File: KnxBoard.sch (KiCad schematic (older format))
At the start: 9 parts, among them J1 SB, J2 KNX, J3 Conn_01x14, J4 Conn_01x02, J5 Conn_01x14, SW1 SW

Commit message: Resistors in 0402
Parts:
- R1: footprint Resistor_SMD:R_0603_1608Metric -> Resistor_SMD:R_0402_1005Metric
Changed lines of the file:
@@
 F 0 "R1" H 2670 1246 50  0000 L CNN
 F 1 "100R" H 2670 1155 50  0000 L CNN
-F 2 "Resistor_SMD:R_0603_1608Metric" V 2530 1200 50  0001 C CNN
-F 3 "https://www.mouser.fr/ProductDetail/Vishay-Dale/CRCW0603100RFKEAC?qs=sGAEpiMZZMvdGkrng054t0DrEhLhGh8gD13mKavhucb20%2FizL9tlHg%3D%3D" H 2600 1200 50  0001 C CNN
+F 2 "Resistor_SMD:R_0402_1005Metric" V 2530 1200 50  0001 C CNN
+F 3 "https://www.mouser.fr/ProductDetail/Vishay-Dale/CRCW0402100RFKEDC?qs=sGAEpiMZZMvdGkrng054t0DrEhLhGh8gJaf4W6KCPV2ghVtyILDy9w%3D%3D" H 2600 1200 50  0001 C CNN
 F 4 "0.09" H 2600 1200 50  0001 C CNN "Price"
 	1    2600 1200

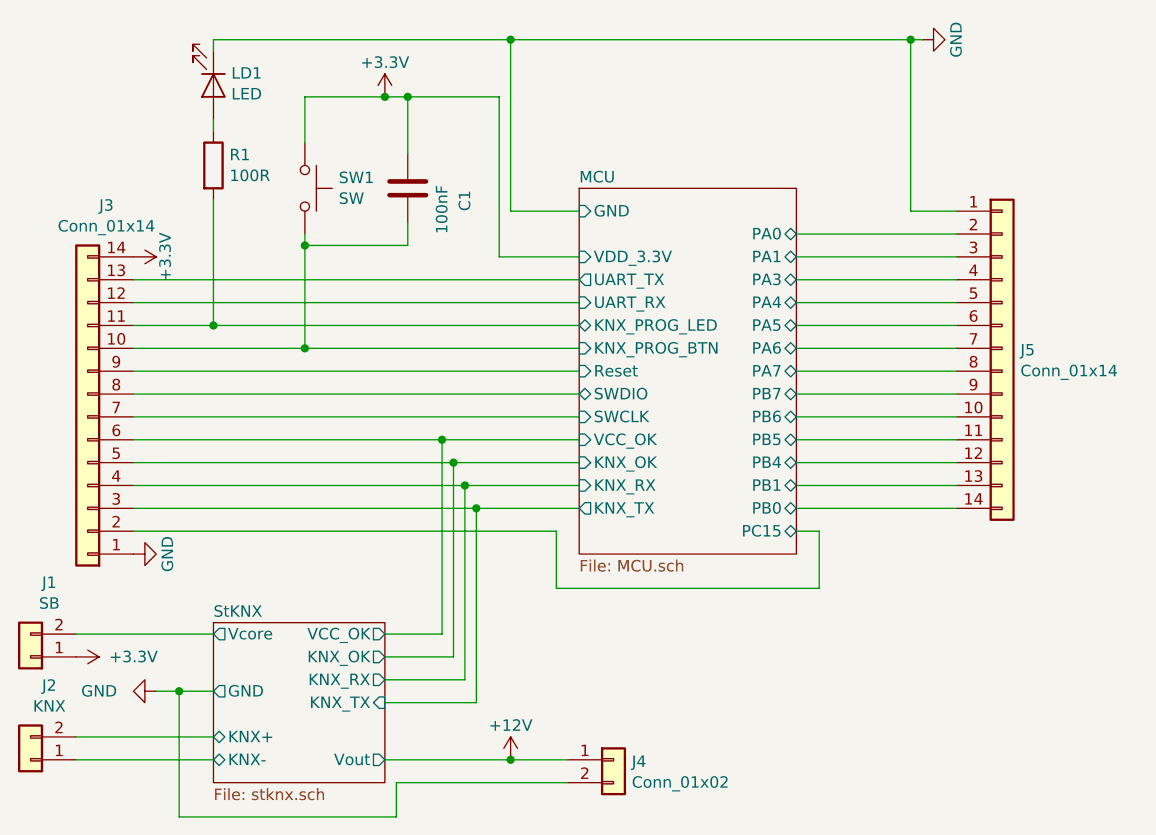
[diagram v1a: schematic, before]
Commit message: Update
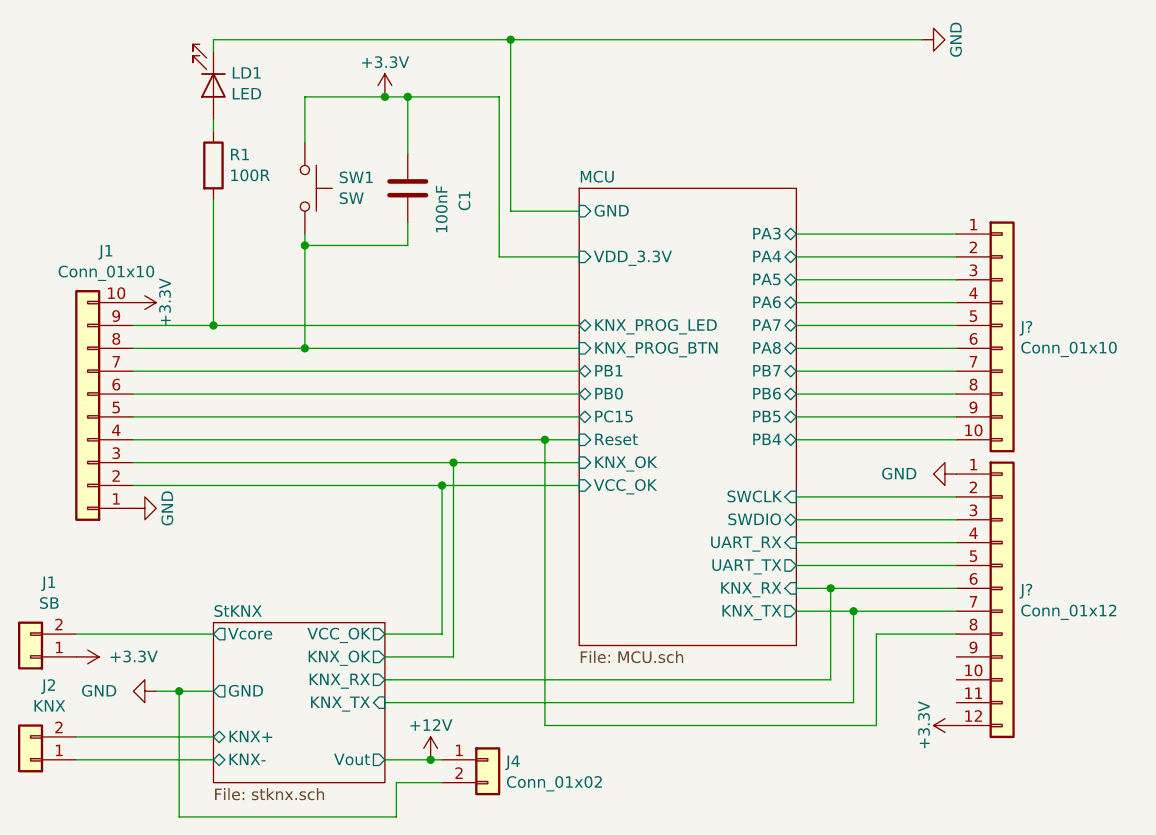
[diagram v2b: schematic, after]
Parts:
- removed J3, J5: Conn_01x14, Connector_PinHeader_2.54mm:PinHeader_1x14_P2.54mm_Vertical, symbol Connector_Generic:Conn_01x14
- added J1: Conn_01x10, Connector_PinHeader_2.54mm:PinHeader_1x14_P2.54mm_Vertical, symbol Connector_Generic:Conn_01x10
- added J?: Conn_01x12, Connector_FFC-FPC:Hirose_FH12-12S-0.5SH_1x12-1MP_P0.50mm_Horizontal, symbol Connector_Generic:Conn_01x12
- added J?: Conn_01x10, symbol Connector_Generic:Conn_01x10
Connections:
- net +3V3: now also J1.10 (Pin_10), J?.12 (Pin_12)
- net GND: now also J1.1 (Pin_1), J?.1 (Pin_1)
- net MCU/KNX_OK: now also J1.3 (Pin_3)
- net MCU/KNX_PROG_BTN: now also J1.8 (Pin_8)
- net MCU/KNX_PROG_LED: now also J1.9 (Pin_9)
- net MCU/KNX_RX: now also J?.6 (Pin_6)
- net MCU/KNX_TX: now also J?.7 (Pin_7)
- net MCU/PA3: now also J?.1 (Pin_1)
- net MCU/PA4: now also J?.2 (Pin_2)
- net MCU/PA5: now also J?.3 (Pin_3)
- net MCU/PA6: now also J?.4 (Pin_4)
- net MCU/PA7: now also J?.5 (Pin_5)
- net MCU/PB0: now also J1.6 (Pin_6)
- net MCU/PB1: now also J1.7 (Pin_7)
- net MCU/PB4: now also J?.10 (Pin_10)
- net MCU/PB5: now also J?.9 (Pin_9)
- net MCU/PB6: now also J?.8 (Pin_8)
- net MCU/PB7: now also J?.7 (Pin_7)
- net MCU/PC15: now also J1.5 (Pin_5)
- net MCU/Reset: now also J1.4 (Pin_4), J?.8 (Pin_8)
- net MCU/SWCLK: now also J?.2 (Pin_2)
- net MCU/SWDIO: now also J?.3 (Pin_3)
- net MCU/UART_RX: now also J?.4 (Pin_4)
- net MCU/UART_TX: now also J?.5 (Pin_5)
- net MCU/VCC_OK: now also J1.2 (Pin_2)
- new net MCU/PA8: J?.6 (Pin_6)
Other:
- moved on the sheet: J4
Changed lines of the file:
@@
 	0    -1   -1   0
 $EndComp
-$Sheet
-S 4200 1300 950  1600
-U 5EC690D9
-F0 "MCU" 50
-F1 "MCU.sch" 50
-F2 "VDD_3.3V" I L 4200 1600 50
-F3 "GND" I L 4200 1400 50
-F4 "PA0" B R 5150 1500 50
-F5 "PA1" B R 5150 1600 50
-F6 "UART_TX" O L 4200 1700 50
-F7 "PA3" B R 5150 1700 50
-F8 "PA4" B R 5150 1800 50
-F9 "PA5" B R 5150 1900 50
-F10 "PA6" B R 5150 2000 50
-F11 "PA7" B R 5150 2100 50
-F12 "KNX_RX" I L 4200 2600 50
-F13 "KNX_TX" O L 4200 2700 50
-F14 "KNX_OK" I L 4200 2500 50
-F15 "VCC_OK" I L 4200 2400 50
-F16 "KNX_PROG_BTN" I L 4200 2000 50
-F17 "SWDIO" B L 4200 2200 50
-F18 "SWCLK" I L 4200 2300 50
-F19 "UART_RX" I L 4200 1800 50
-F20 "PB7" B R 5150 2200 50
-F21 "PB6" B R 5150 2300 50
-F22 "PB5" B R 5150 2400 50
-F23 "PB4" B R 5150 2500 50
-F24 "KNX_PROG_LED" B L 4200 1900 50
-F25 "PB1" B R 5150 2600 50
-F26 "PB0" B R 5150 2700 50
-F27 "PC15" B R 5150 2800 50
-F28 "Reset" I L 4200 2100 50
-$EndSheet
-Wire Wire Line
-	4200 1700 2250 1700
-Wire Wire Line
-	4200 1800 2250 1800
 $Comp
 L Device:LED LD1
@@
 $EndComp
 Wire Wire Line
-	5650 1400 5650 650
-Wire Wire Line
-	5650 650  3900 650
-Wire Wire Line
 	4200 1400 3900 1400
 Wire Wire Line
 	3900 1400 3900 650
 Connection ~ 3900 650
-Wire Wire Line
-	5650 650  5700 650
-Connection ~ 5650 650
 $Comp
 L Device:R R1
@@
 Wire Wire Line
 	3000 1550 3000 2000
-Wire Wire Line
-	4200 2100 2250 2100
-Wire Wire Line
-	4200 2200 2250 2200
-Wire Wire Line
-	4200 2300 2250 2300
 $Comp
 L power:+12V #PWR03
 U 1 1 5EE9DBC4
-P 3900 3800
-F 0 "#PWR03" H 3900 3650 50  0001 C CNN
-F 1 "+12V" H 3900 3950 50  0000 C CNN
-F 2 "" H 3900 3800 50  0000 C CNN
-F 3 "" H 3900 3800 50  0000 C CNN
-	1    3900 3800
+P 3550 3800
+F 0 "#PWR03" H 3550 3650 50  0001 C CNN
+F 1 "+12V" H 3550 3950 50  0000 C CNN
+F 2 "" H 3550 3800 50  0000 C CNN
+F 3 "" H 3550 3800 50  0000 C CNN
+	1    3550 3800
 	1    0    0    -1
 $EndComp
@@
 L power:GND #PWR01
 U 1 1 50827367
-P 2250 2900
-F 0 "#PWR01" H 2250 2650 50  0001 C CNN
-F 1 "GND" H 2250 2750 50  0000 C CNN
-F 2 "" H 2250 2900 50  0000 C CNN
-F 3 "" H 2250 2900 50  0000 C CNN
-	1    2250 2900
+P 2250 2700
+F 0 "#PWR01" H 2250 2450 50  0001 C CNN
+F 1 "GND" H 2250 2550 50  0000 C CNN
+F 2 "" H 2250 2700 50  0000 C CNN
+F 3 "" H 2250 2700 50  0000 C CNN
+	1    2250 2700
 	0    -1   -1   0
 $EndComp
-$Comp
-L Connector_Generic:Conn_01x14 J3
-U 1 1 5EC2ECF7
-P 2050 2300
-F 0 "J3" H 1968 1375 50  0000 C CNN
-F 1 "Conn_01x14" H 1968 1466 50  0000 C CNN
-F 2 "Connector_PinHeader_2.54mm:PinHeader_1x14_P2.54mm_Vertical" H 2050 2300 50  0001 C CNN
-F 3 "~" H 2050 2300 50  0001 C CNN
-	1    2050 2300
-	-1   0    0    1
-$EndComp
-Wire Wire Line
-	5150 2200 5850 2200
-Wire Wire Line
-	5150 2100 5850 2100
 Wire Wire Line
 	5150 2000 5850 2000
@@
 	5150 1500 5850 1500
 Wire Wire Line
-	5150 2600 5850 2600
-Wire Wire Line
-	5150 2500 5850 2500
-Wire Wire Line
-	5150 2400 5850 2400
-Wire Wire Line
-	5150 2300 5850 2300
-Wire Wire Line
-	5850 1400 5650 1400
-$Comp
-L Connector_Generic:Conn_01x14 J5
-U 1 1 5EC2D487
-P 6050 2000
-F 0 "J5" H 6130 1992 50  0000 L CNN
-F 1 "Conn_01x14" H 6130 1901 50  0000 L CNN
-F 2 "Connector_PinHeader_2.54mm:PinHeader_1x14_P2.54mm_Vertical" H 6050 2000 50  0001 C CNN
-F 3 "~" H 6050 2000 50  0001 C CNN
-	1    6050 2000
-	1    0    0    -1
-$EndComp
-Wire Wire Line
-	5850 2700 5150 2700
-Wire Wire Line
 	3350 3250 3600 3250
 Wire Wire Line
 	3350 3350 3650 3350
-Wire Wire Line
-	3350 3450 3700 3450
-Wire Wire Line
-	3350 3550 3750 3550
-Wire Wire Line
-	3600 2400 2250 2400
-Wire Wire Line
-	3600 2400 3600 3250
-Wire Wire Line
-	3600 2400 4200 2400
-Connection ~ 3600 2400
-Wire Wire Line
-	2250 2600 3700 2600
-Wire Wire Line
-	2250 2700 3750 2700
-Wire Wire Line
-	3750 2700 3750 3550
-Connection ~ 3750 2700
-Wire Wire Line
-	3750 2700 4200 2700
-Wire Wire Line
-	3700 3450 3700 2600
-Connection ~ 3700 2600
-Wire Wire Line
-	3700 2600 4200 2600
-Wire Wire Line
-	2250 2500 3650 2500
-Wire Wire Line
-	3650 3350 3650 2500
-Connection ~ 3650 2500
-Wire Wire Line
-	3650 2500 4200 2500
 $Comp
 L Connector_Generic:Conn_01x02 J4
 U 1 1 5EEFA76B
-P 4350 3800
-F 0 "J4" H 4430 3792 50  0000 L CNN
-F 1 "Conn_01x02" H 4430 3701 50  0000 L CNN
-F 2 "Connector_PinHeader_2.54mm:PinHeader_1x02_P2.54mm_Vertical" H 4350 3800 50  0001 C CNN
-F 3 "~" H 4350 3800 50  0001 C CNN
-	1    4350 3800
-	1    0    0    -1
-$EndComp
-Wire Wire Line
-	3350 3800 3900 3800
-Connection ~ 3900 3800
-Wire Wire Line
-	3900 3800 4150 3800
+P 3800 3800
+F 0 "J4" H 3880 3792 50  0000 L CNN
+F 1 "Conn_01x02" H 3880 3701 50  0000 L CNN
+F 2 "Connector_PinHeader_2.54mm:PinHeader_1x02_P2.54mm_Vertical" H 3800 3800 50  0001 C CNN
+F 3 "~" H 3800 3800 50  0001 C CNN
+	1    3800 3800
+	1    0    0    -1
+$EndComp
 Wire Wire Line
 	2350 3500 2450 3500
-Wire Wire Line
-	4150 3900 3400 3900
 Wire Wire Line
 	3400 3900 3400 4050
@@
 Wire Wire Line
 	2450 3500 2600 3500
-Wire Wire Line
-	5150 2800 5250 2800
-Wire Wire Line
-	5250 2800 5250 3050
-Wire Wire Line
-	5250 3050 4100 3050
-Wire Wire Line
-	4100 3050 4100 2800
-Wire Wire Line
-	4100 2800 2250 2800
 $Comp
 L power:+3.3V #PWR3.3V01
@@
 L power:+3.3V #PWR3.3V02
 U 1 1 50827375
-P 2250 1600
-F 0 "#PWR3.3V02" H 2250 1450 50  0001 C CNN
-F 1 "+3.3V" H 2250 1740 50  0000 C CNN
-F 2 "" H 2250 1600 50  0000 C CNN
-F 3 "" H 2250 1600 50  0000 C CNN
-	1    2250 1600
+P 2250 1800
+F 0 "#PWR3.3V02" H 2250 1650 50  0001 C CNN
+F 1 "+3.3V" H 2250 1940 50  0000 C CNN
+F 2 "" H 2250 1800 50  0000 C CNN
+F 3 "" H 2250 1800 50  0000 C CNN
+	1    2250 1800
 	0    1    1    0
 $EndComp
@@
 Wire Wire Line
 	2000 3800 2600 3800
+$Comp
+L Connector_Generic:Conn_01x12 J?
+U 1 1 5FF7779A
+P 6050 3050
+F 0 "J?" H 6130 3042 50  0000 L CNN
+F 1 "Conn_01x12" H 6130 2951 50  0000 L CNN
+F 2 "Connector_FFC-FPC:Hirose_FH12-12S-0.5SH_1x12-1MP_P0.50mm_Horizontal" H 6050 3050 50  0001 C CNN
+F 3 "https://www.mouser.fr/ProductDetail/Hirose-Connector/FH12-12S-05SH55/?qs=Ux3WWAnHpjA1i1nP49r1%2FQ%3D%3D" H 6050 3050 50  0001 C CNN
+	1    6050 3050
+	1    0    0    -1
+$EndComp
+$Comp
+L power:GND #PWR?
+U 1 1 5FF97B18
+P 5850 2550
+F 0 "#PWR?" H 5850 2300 50  0001 C CNN
+F 1 "GND" V 5850 2300 50  0000 C CNN
+F 2 "" H 5850 2550 50  0000 C CNN
+F 3 "" H 5850 2550 50  0000 C CNN
+	1    5850 2550
+	0    1    1    0
+$EndComp
+$Comp
+L power:+3.3V #PWR3.3V?
+U 1 1 5FF982D6
+P 5850 3650
+F 0 "#PWR3.3V?" H 5850 3500 50  0001 C CNN
+F 1 "+3.3V" H 5850 3790 50  0000 C CNN
+F 2 "" H 5850 3650 50  0000 C CNN
+F 3 "" H 5850 3650 50  0000 C CNN
+	1    5850 3650
+	0    -1   -1   0
+$EndComp
+$Comp
+L Connector_Generic:Conn_01x10 J1
+U 1 1 5FFB9488
+P 2050 2300
+F 0 "J1" H 1968 1575 50  0000 C CNN
+F 1 "Conn_01x10" H 1968 1666 50  0000 C CNN
+F 2 "Connector_PinHeader_2.54mm:PinHeader_1x14_P2.54mm_Vertical" H 2050 2300 50  0001 C CNN
+F 3 "~" H 2050 2300 50  0001 C CNN
+	1    2050 2300
+	-1   0    0    1
+$EndComp
+Wire Wire Line
+	3900 650  5700 650
+$Comp
+L Connector_Generic:Conn_01x10 J?
+U 1 1 5FFD98D6
+P 6050 1900
+F 0 "J?" H 6130 1892 50  0000 L CNN
+F 1 "Conn_01x10" H 6130 1801 50  0000 L CNN
+F 2 "" H 6050 1900 50  0001 C CNN
+F 3 "~" H 6050 1900 50  0001 C CNN
+	1    6050 1900
+	1    0    0    -1
+$EndComp
+Wire Wire Line
+	5150 2100 5850 2100
+Wire Wire Line
+	5150 2200 5850 2200
+Wire Wire Line
+	5150 2300 5850 2300
+Wire Wire Line
+	5150 2400 5850 2400
+$Sheet
+S 4200 1300 950  2000
+U 5EC690D9
+F0 "MCU" 50
+F1 "MCU.sch" 50
+F2 "VDD_3.3V" I L 4200 1600 50
+F3 "GND" I L 4200 1400 50
+F4 "UART_TX" O R 5150 2950 50
+F5 "PA3" B R 5150 1500 50
+F6 "PA4" B R 5150 1600 50
+F7 "PA5" B R 5150 1700 50
+F8 "PA6" B R 5150 1800 50
+F9 "PA7" B R 5150 1900 50
+F10 "KNX_RX" I R 5150 3050 50
+F11 "KNX_TX" O R 5150 3150 50
+F12 "KNX_OK" I L 4200 2500 50
+F13 "VCC_OK" I L 4200 2600 50
+F14 "KNX_PROG_BTN" I L 4200 2000 50
+F15 "SWDIO" B R 5150 2750 50
+F16 "SWCLK" I R 5150 2650 50
+F17 "UART_RX" I R 5150 2850 50
+F18 "PB7" B R 5150 2100 50
+F19 "PB6" B R 5150 2200 50
+F20 "PB5" B R 5150 2300 50
+F21 "PB4" B R 5150 2400 50
+F22 "KNX_PROG_LED" B L 4200 1900 50
+F23 "PB1" B L 4200 2100 50
+F24 "PB0" B L 4200 2200 50
+F25 "PC15" B L 4200 2300 50
+F26 "Reset" I L 4200 2400 50
+F27 "PA8" B R 5150 2000 50
+$EndSheet
+Wire Wire Line
+	2250 2100 4200 2100
+Wire Wire Line
+	2250 2200 4200 2200
+Wire Wire Line
+	2250 2300 4200 2300
+Wire Wire Line
+	2250 2400 4050 2400
+Wire Wire Line
+	2250 2500 3650 2500
+Wire Wire Line
+	2250 2600 3600 2600
+Wire Wire Line
+	3600 3250 3600 2600
+Connection ~ 3600 2600
+Wire Wire Line
+	3600 2600 4200 2600
+Connection ~ 3650 2500
+Wire Wire Line
+	3650 2500 4200 2500
+Wire Wire Line
+	3650 2500 3650 3350
+Wire Wire Line
+	5150 2650 5850 2650
+Wire Wire Line
+	5150 2750 5850 2750
+Wire Wire Line
+	5150 2850 5850 2850
+Wire Wire Line
+	5150 2950 5850 2950
+Wire Wire Line
+	5150 3050 5300 3050
+Wire Wire Line
+	5150 3150 5400 3150
+Wire Wire Line
+	5300 3450 5300 3050
+Wire Wire Line
+	3350 3450 5300 3450
+Connection ~ 5300 3050
+Wire Wire Line
+	5300 3050 5850 3050
+Wire Wire Line
+	5400 3550 5400 3150
+Wire Wire Line
+	3350 3550 5400 3550
+Connection ~ 5400 3150
+Wire Wire Line
+	5400 3150 5850 3150
+Wire Wire Line
+	3600 3900 3400 3900
+Wire Wire Line
+	3550 3800 3600 3800
+Wire Wire Line
+	3350 3800 3550 3800
+Connection ~ 3550 3800
+Wire Wire Line
+	4050 2400 4050 3650
+Wire Wire Line
+	4050 3650 5500 3650
+Wire Wire Line
+	5500 3650 5500 3250
+Wire Wire Line
+	5500 3250 5850 3250
+Connection ~ 4050 2400
+Wire Wire Line
+	4050 2400 4200 2400
 $EndSCHEMATC
